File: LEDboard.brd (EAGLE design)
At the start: 72 x 72 mm, 321 parts, among them J1 JTAG, U1 IS31FL3741_QFN60, U2 IS31FL3741_QFN60, U3 ATSAMD21E, U4 TPS61090RSAR, U5 MCP73831T-2ACI/OT, Y1 32.768kHz

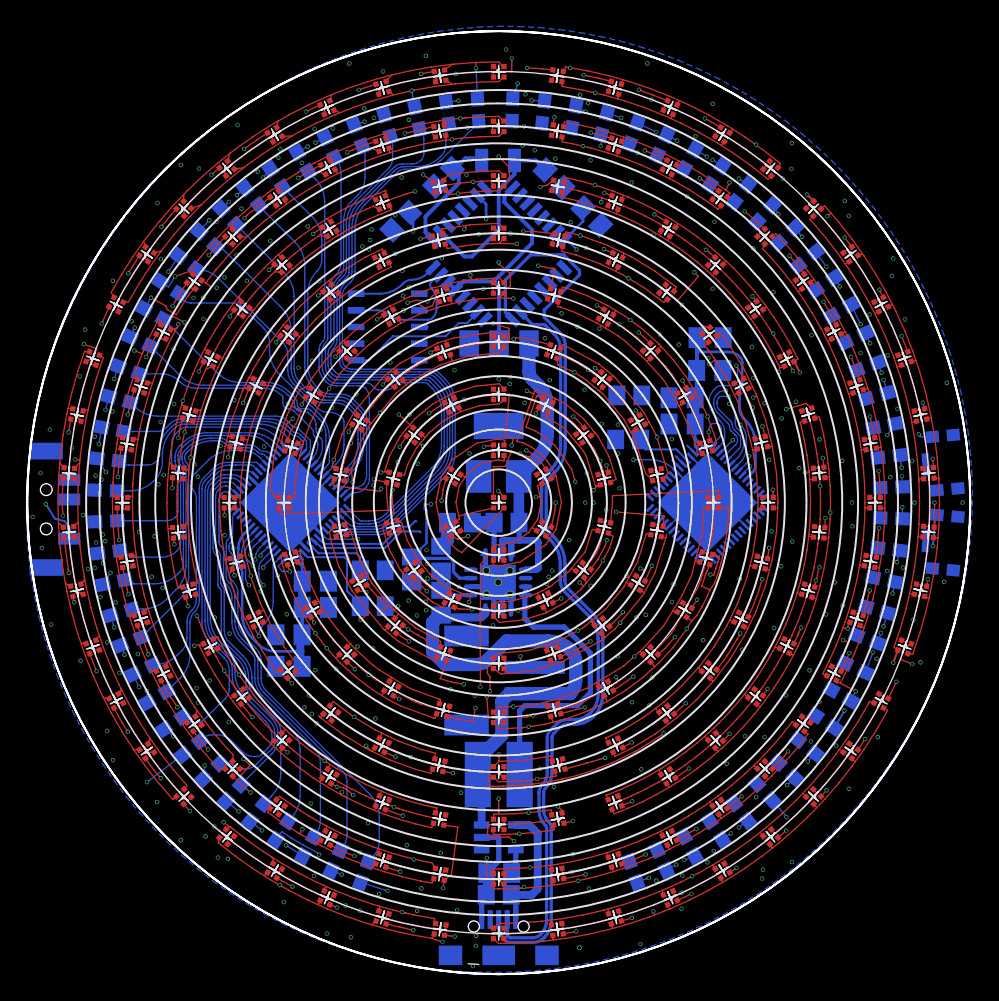
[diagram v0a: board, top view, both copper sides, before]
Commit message: complete
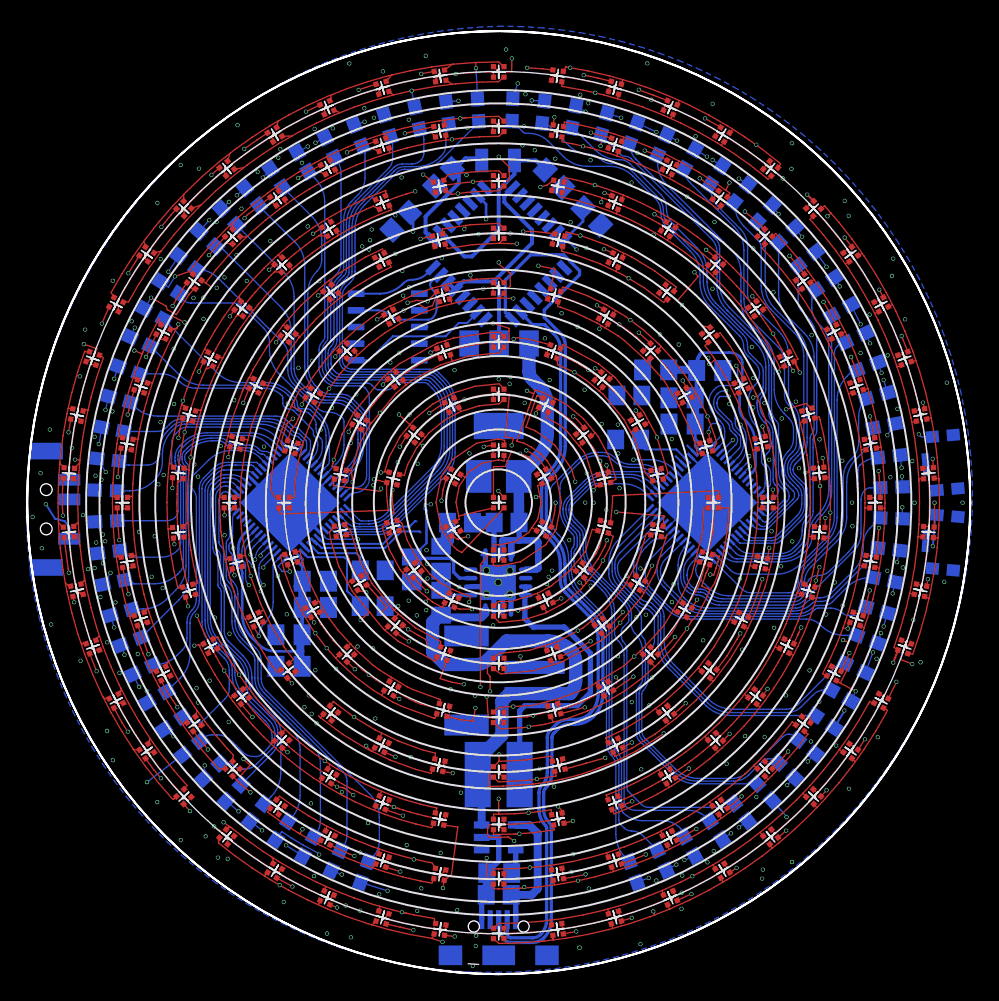
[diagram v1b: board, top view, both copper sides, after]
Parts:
- moved C16 4.83 mm to (12.0, 10.1), turned to 0 degrees
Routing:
- net N$13: track 0.00 -> 40.6 mm
- net N$14: track 0.00 -> 40.1 mm
- net N$20: track 0.00 -> 39.9 mm
- net N$15: track 0.00 -> 39.3 mm
- net N$19: track 0.00 -> 39.1 mm
- net N$72: track 0.00 -> 38.5 mm
- net N$71: track 0.00 -> 37.1 mm
- net N$21: track 0.00 -> 36.8 mm
- net N$70: track 0.00 -> 36.2 mm
- net N$69: track 0.00 -> 35.7 mm
- net N$68: track 0.00 -> 34.7 mm
- net N$26: track 0.00 -> 34.3 mm
- net N$67: track 0.00 -> 34.3 mm
- net N$66: track 0.00 -> 33.3 mm
- net N$65: track 0.00 -> 33.1 mm
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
